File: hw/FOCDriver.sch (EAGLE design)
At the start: 100 parts, among them U1 IX4428N, U2 IX4428N, U3 IX4428N, U4 IRF9389TRPBF, U5 IRF9389TRPBF, U6 IRF9389TRPBF, U7 LM27313XMF, U8 LM358N, U9 LM358N

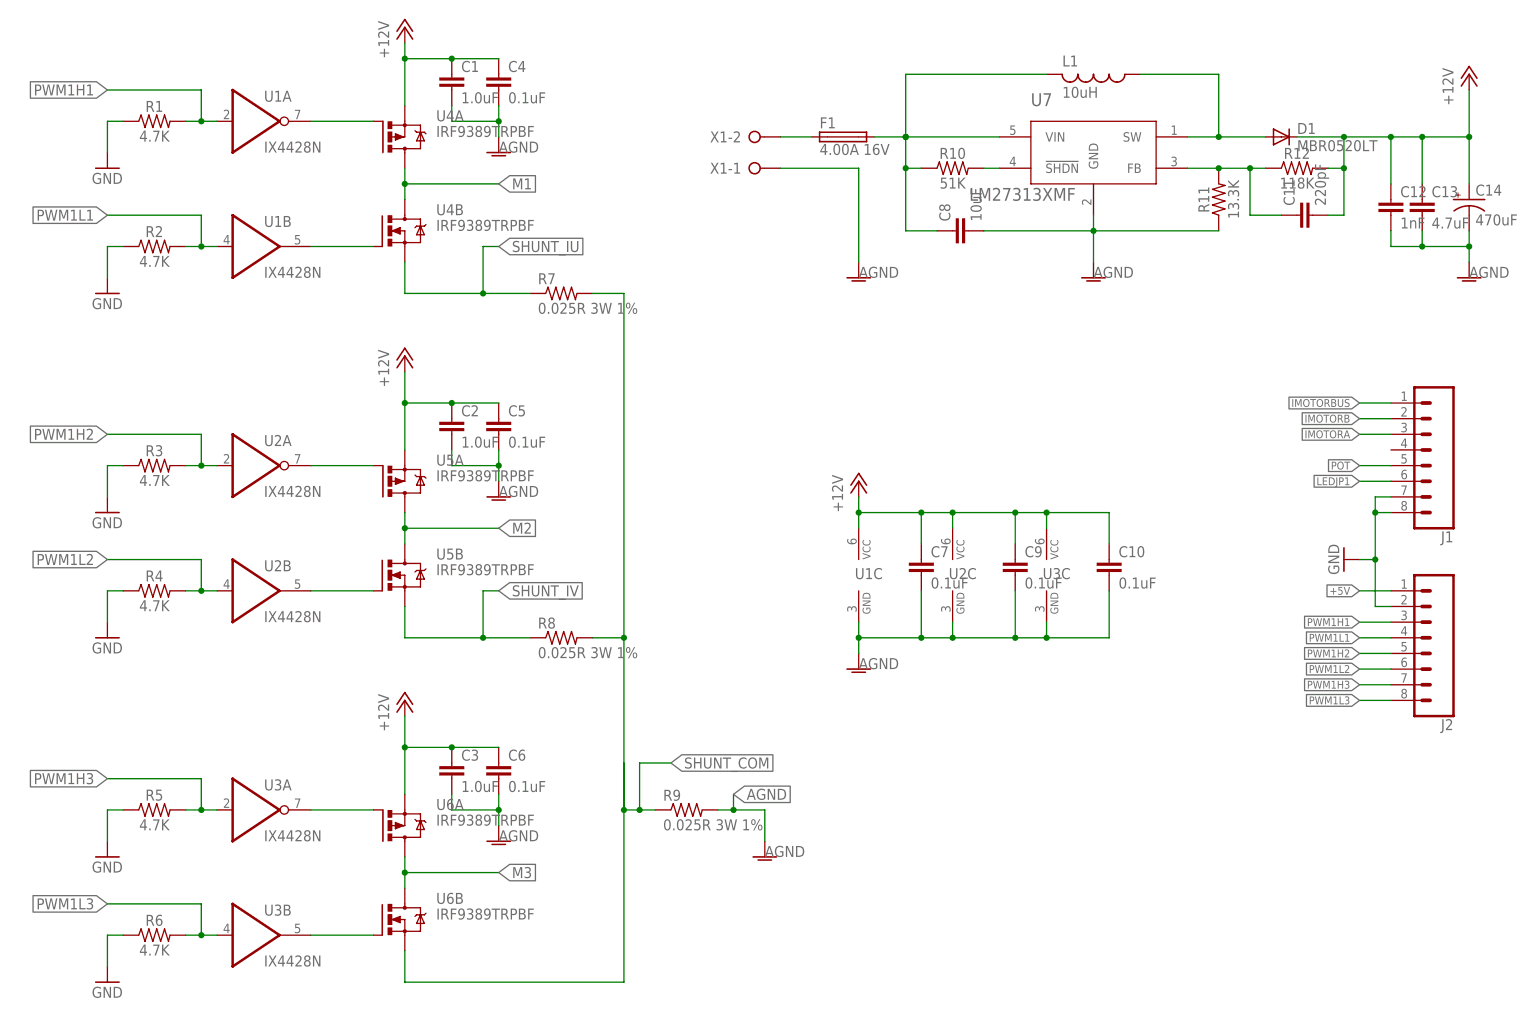
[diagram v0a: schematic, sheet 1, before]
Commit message: trans
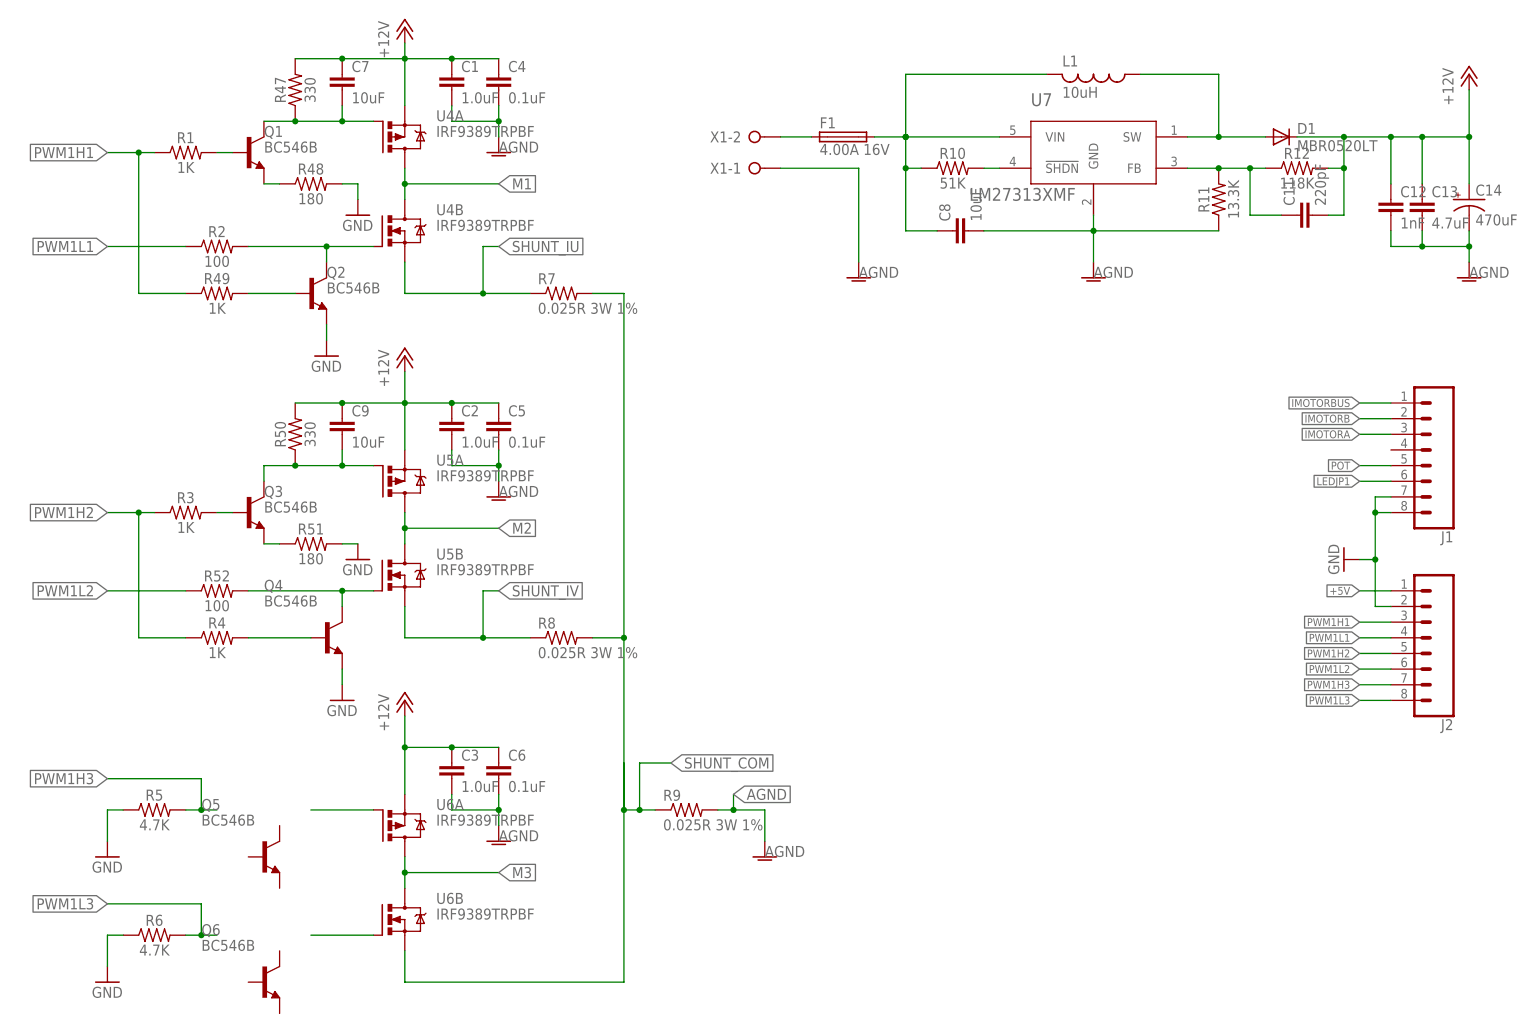
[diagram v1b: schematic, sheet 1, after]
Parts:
- removed C10: 0.1uF, SparkFun-Capacitors:1.0UF-0805-25V-10%
- removed U1, U2, U3: IX4428N, IX4428N:IX4428N
- added Q1, Q2, Q3, Q4, Q5, Q6: BC546B, transistor-npn:BC546B
- added R47, R50: 330, SparkFun-Resistors:RESISTOR0805
- added R48, R51: 180, SparkFun-Resistors:RESISTOR0805
- added R49: 1K, SparkFun-Resistors:RESISTOR0805
- added R52: 100, SparkFun-Resistors:RESISTOR0805
- C7, C9: value 0.1uF -> 10uF
- R1, R3, R4: value 4.7K -> 1K
- R2: value 4.7K -> 100
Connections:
- new net N$28: Q1.E, R48.1
- new net N$30: Q1.B, R1.2
- new net N$32: Q2.B, R49.2
- new net N$39: Q3.B, R3.2
- new net N$40: Q3.E, R51.1
- new net N$41: Q4.B, R4.2
- net +12V: now also R47.2, R50.2; no longer C10.1, U1C.VCC, U2C.VCC, U3C.VCC
- net AGND: no longer C10.2, C7.2, C9.2, U1C.GND, U2C.GND, U3C.GND
- net GND: now also Q2.E, Q4.E, R48.2, R51.2; no longer R1.1, R2.1, R3.1, R4.1
- net N$10: now also C7.2, Q1.C, R47.1; no longer U1A.O
- net N$3: no longer U3B.O
- net N$6: no longer U3A.O
- net N$7: now also Q4.C, R52.2; no longer U2B.O
- net N$8: now also C9.2, Q3.C, R50.1; no longer U2A.O
- net N$9: now also Q2.C, R2.2; no longer U1B.O
- net PWM1H1: now also R1.1, R49.1; no longer R1.2, U1A.I
- net PWM1H2: now also R3.1, R4.1; no longer R3.2, U2A.I
- net PWM1H3: no longer U3A.I
- net PWM1L1: now also R2.1; no longer R2.2, U1B.I
- net PWM1L2: now also R52.1; no longer R4.2, U2B.I
- net PWM1L3: no longer U3B.I
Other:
- moved on the sheet: C7, C9, R1, R2, R3, R4
